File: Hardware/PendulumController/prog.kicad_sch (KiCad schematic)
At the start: 14 parts, among them J401 USB_B_Micro, J402 PROG, U401 FT232RL

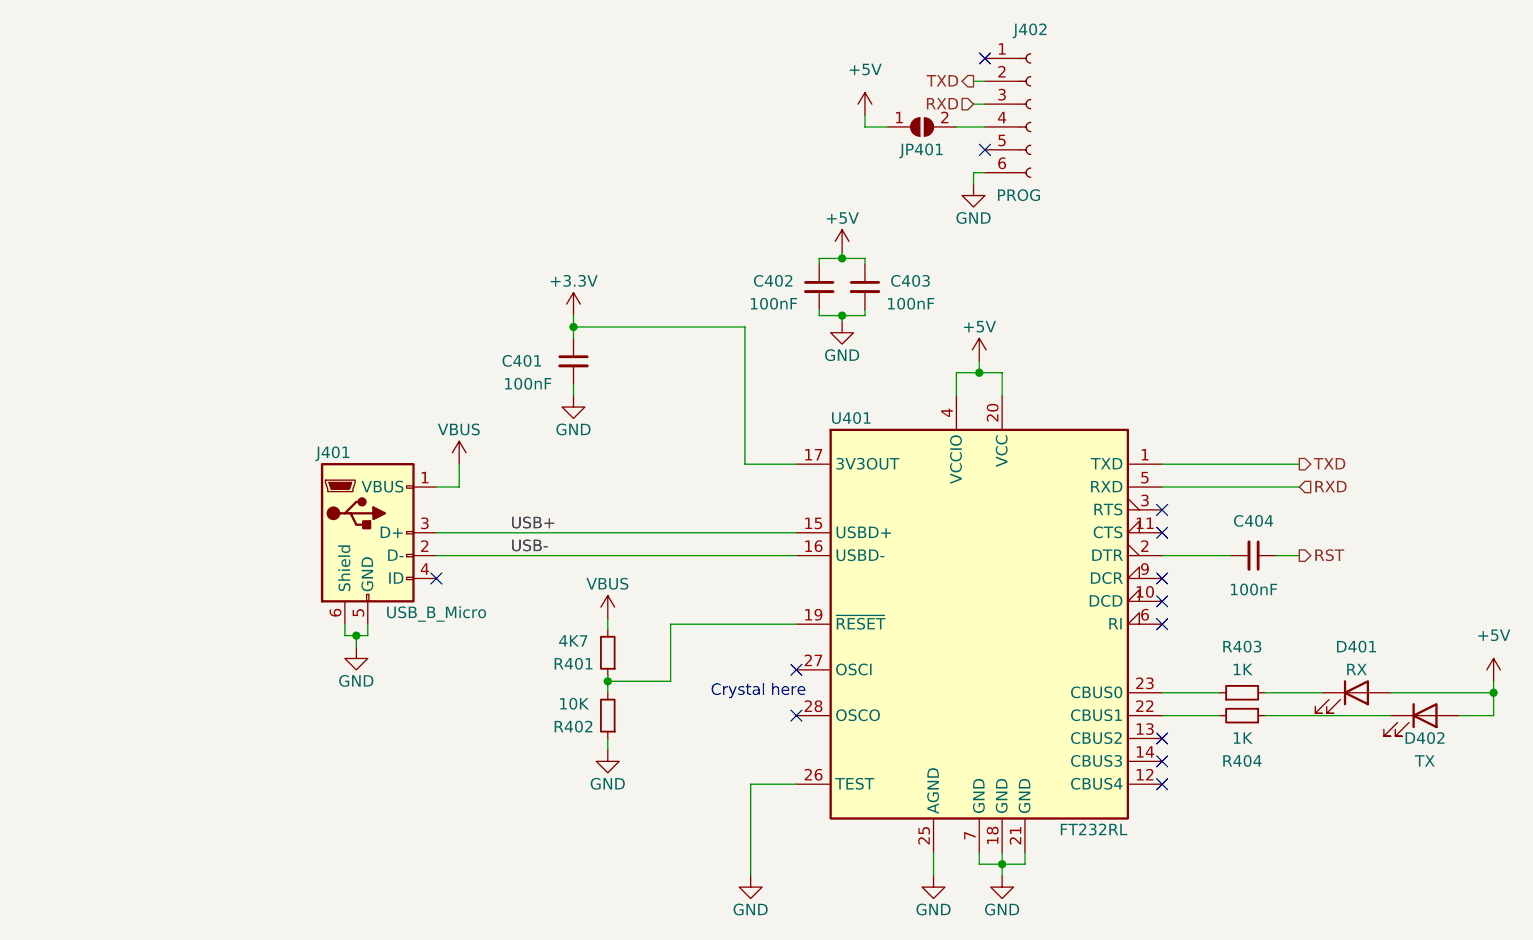
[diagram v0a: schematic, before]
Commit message: USB C!
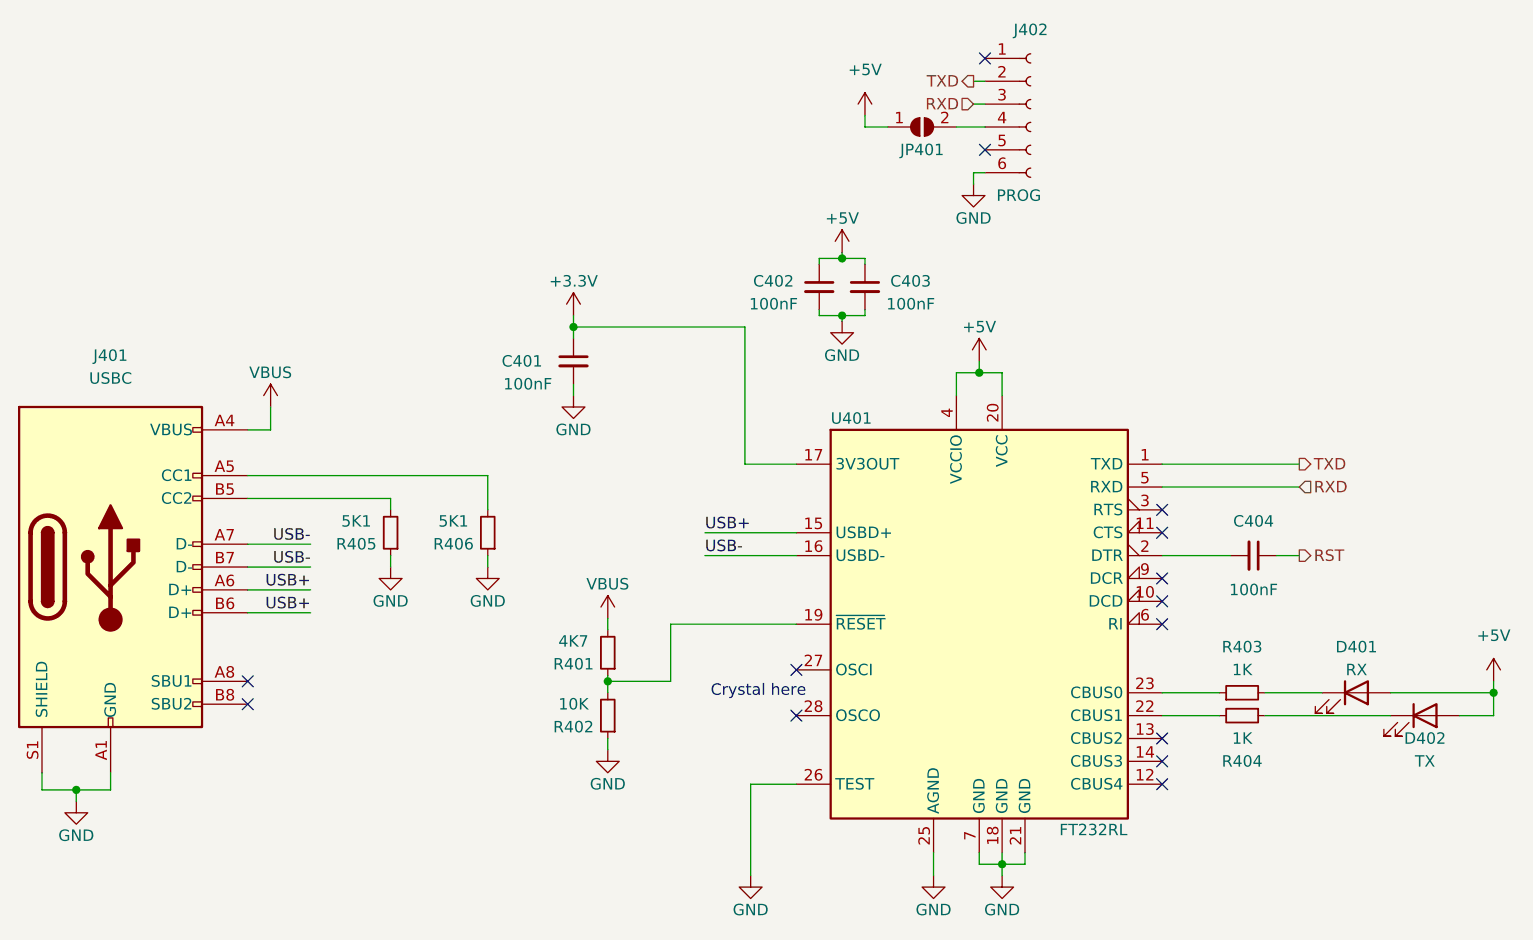
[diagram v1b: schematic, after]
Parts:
- removed J401: USB_B_Micro, Connector_USB:USB_Mini-B_Lumberg_2486_01_Horizontal, symbol Connector:USB_B_Micro
- added J401: USBC, symbol Connector:USB_C_Receptacle_USB2.0
- added R405, R406: 5K1, Resistor_SMD:R_0805_2012Metric, symbol Device:R_Small
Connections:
- net GND: now also J401.A1 (GND), J401.A12 (GND), J401.B1 (GND), J401.B12 (GND), J401.S1 (SHIELD), R405.1, R406.1
- net USB+: now also J401.A6 (D+), J401.B6 (D+)
- net USB-: now also J401.A7 (D-), J401.B7 (D-)
- net VBUS: now also J401.A4 (VBUS), J401.A9 (VBUS), J401.B4 (VBUS), J401.B9 (VBUS)
- new net: J401.B5 (CC2), R405.2
- new net: J401.A5 (CC1), R406.2
- no-connect marks 13 -> 14
